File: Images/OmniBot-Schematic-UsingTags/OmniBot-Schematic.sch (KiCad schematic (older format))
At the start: 13 parts

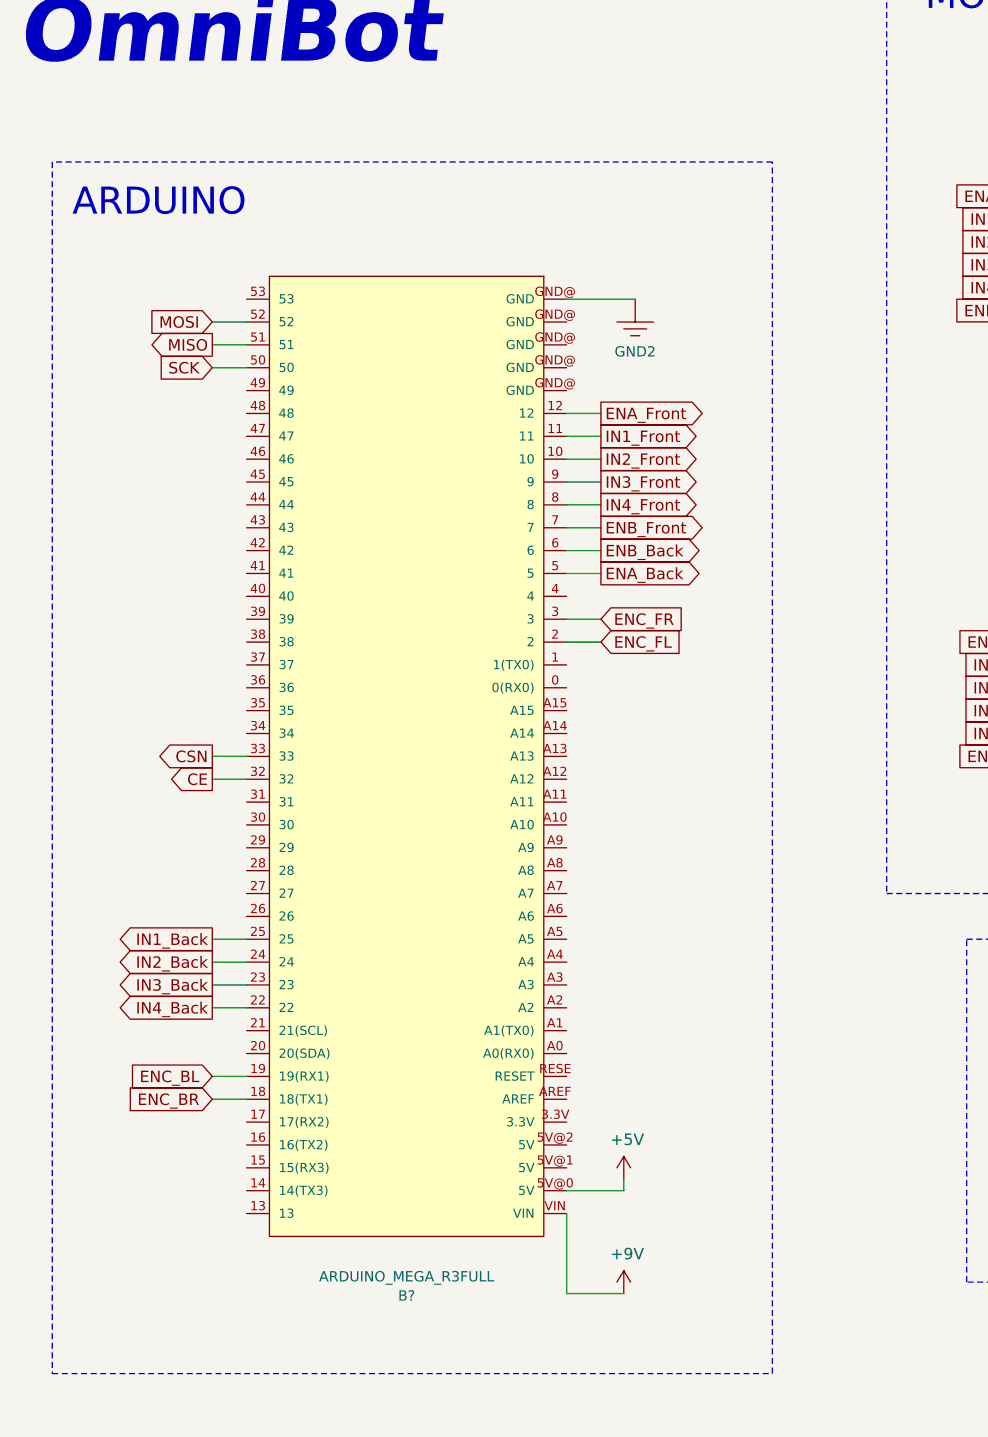
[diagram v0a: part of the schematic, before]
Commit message: Update schematic and code
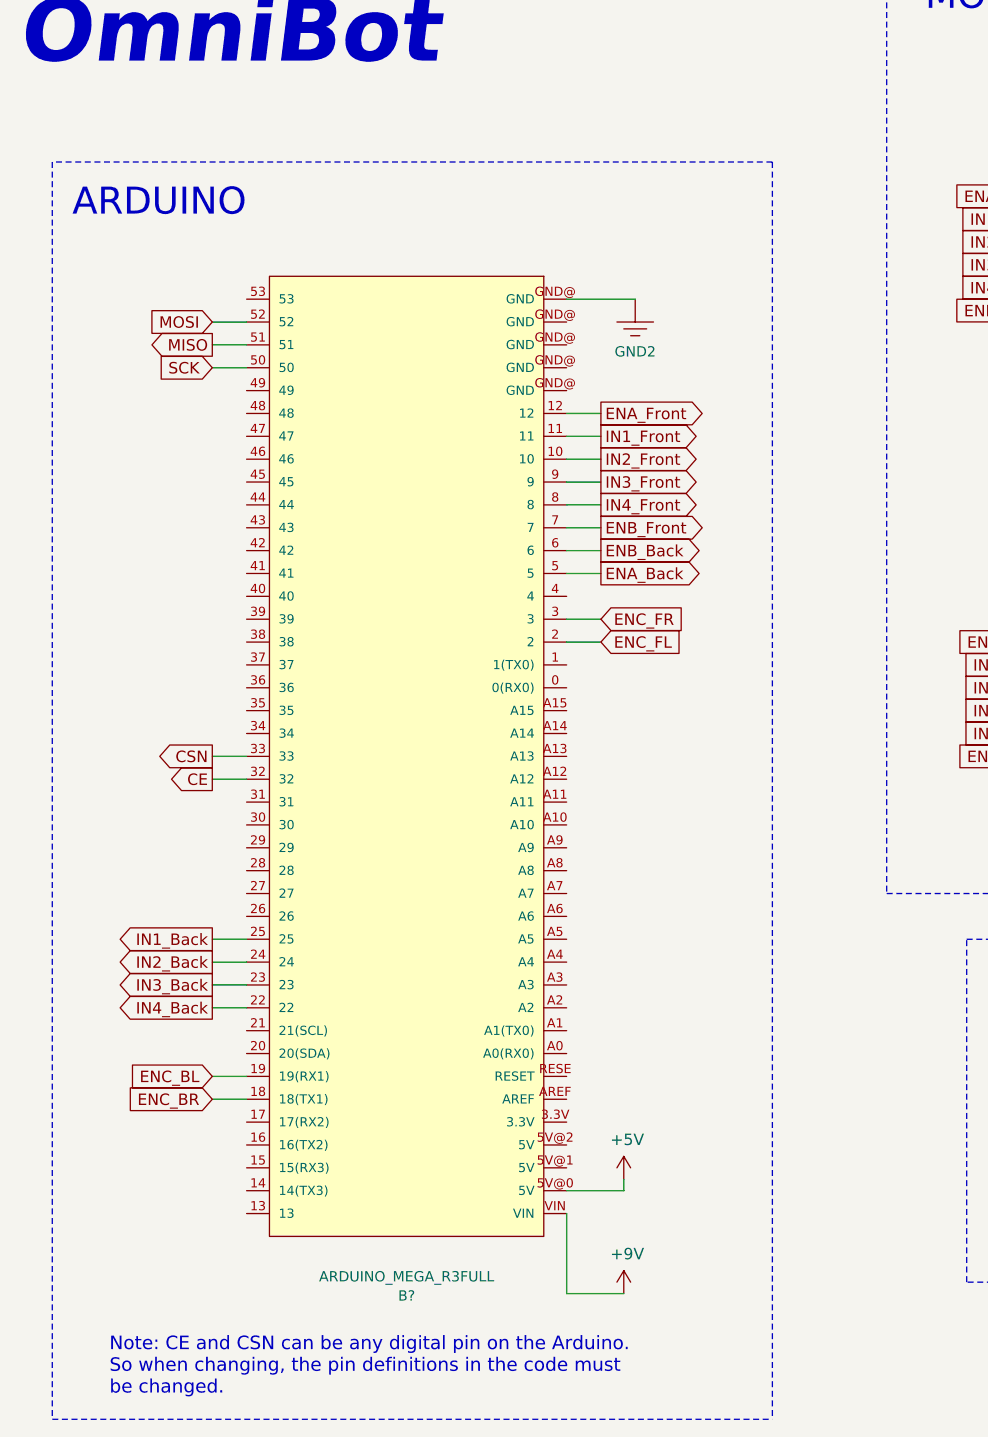
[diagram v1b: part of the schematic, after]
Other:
- note added: "Note: CE and CSN can be any digital pin on the Arduino. \nSo when changing, the pin definitions in the code must \nbe changed."
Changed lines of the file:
@@
 	3250 6600 3500 6600
 Wire Notes Line
-	1000 6950 4150 6950
-Wire Notes Line
-	4150 6950 4150 1650
+	1000 7150 4150 7150
 Wire Notes Line
 	4150 1650 1000 1650
-Wire Notes Line
-	1000 1650 1000 6950
 Wire Notes Line
 	4650 4850 8200 4850
@@
 Wire Wire Line
 	5450 5950 6350 5950
+Text Notes 1250 7050 0    59   ~ 0
+Note: CE and CSN can be any digital pin on the Arduino. \nSo when changing, the pin definitions in the code must \nbe changed.
+Wire Notes Line
+	4150 1650 4150 7150
+Wire Notes Line
+	1000 1650 1000 7150
 $EndSCHEMATC
